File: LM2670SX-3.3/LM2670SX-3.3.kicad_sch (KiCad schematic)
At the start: 2 parts, among them IC1 LM2670SX-3.3_NOPB, J1 Conn_01x03

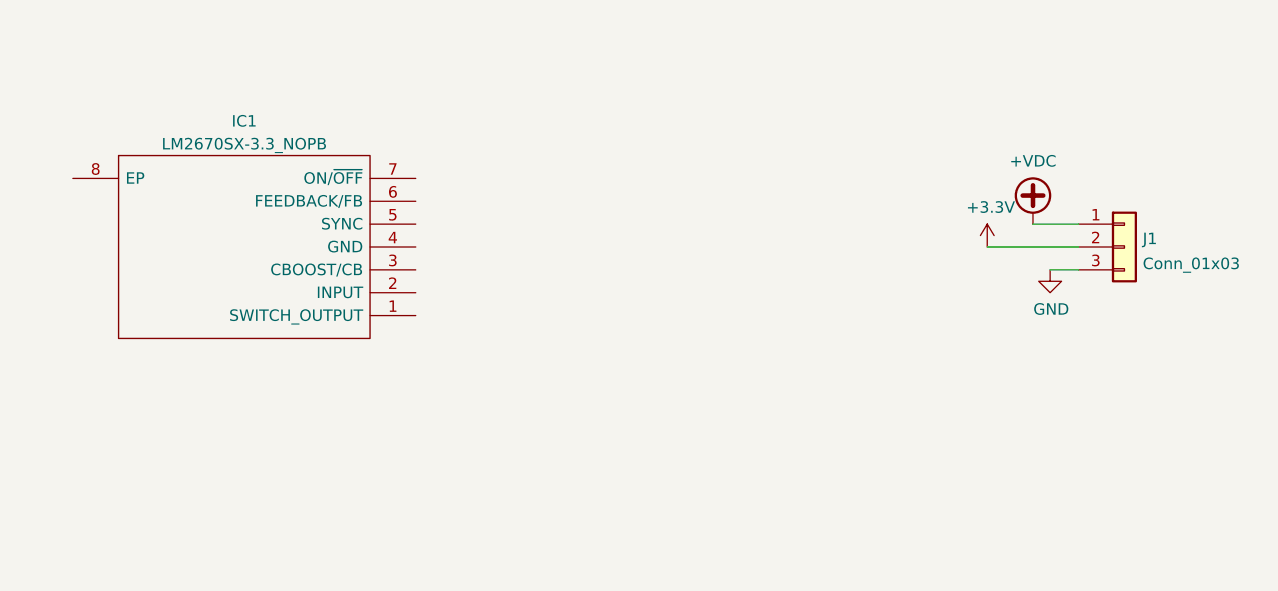
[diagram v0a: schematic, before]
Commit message: finished and drc'ed
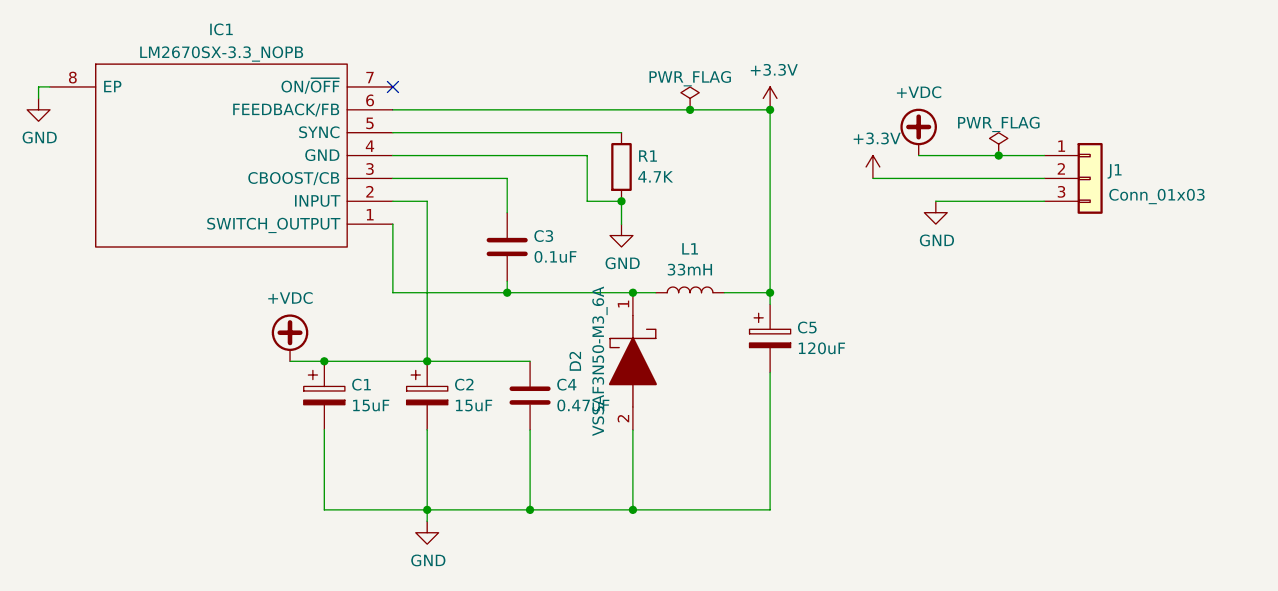
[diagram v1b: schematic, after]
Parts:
- added C1, C2: 15uF, Capacitor_THT:CP_Radial_D5.0mm_P2.50mm, symbol Device:CP
- added C3: 0.1uF, Capacitor_SMD:C_0603_1608Metric_Pad1.08x0.95mm_HandSolder, symbol Device:C
- added C4: 0.47uF, Capacitor_SMD:C_0603_1608Metric_Pad1.08x0.95mm_HandSolder, symbol Device:C
- added C5: 120uF, Capacitor_THT:CP_Radial_D8.0mm_P5.00mm, symbol Device:CP
- added D2: VSSAF3N50-M3_6A, SODFL5226X100N, symbol SamacSys_Parts:VSSAF3N50-M3_6A
- added L1: 33mH, Inductor_THT:L_Axial_L9.5mm_D4.0mm_P15.24mm_Horizontal_Fastron_SMCC, symbol Device:L
- added R1: 4.7K, Resistor_SMD:R_0612_1632Metric_Pad1.18x3.40mm_HandSolder, symbol Device:R
- IC1: footprint LM2670SX33NOPB -> SamacSys_Parts:LM2670SX33NOPB
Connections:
- net +3V3: now also IC1.6 (FEEDBACK/FB), C5.1, L1.2
- net +VDC: now also IC1.2 (INPUT), C1.1, C2.1, C4.1
- net GND: now also IC1.4 (GND), IC1.8 (EP), C1.2, C2.2, C4.2, C5.2, D2.2, R1.2
- net at IC1.1 (SWITCH_OUTPUT): now also C3.2, D2.1, L1.1
- net at IC1.3 (CBOOST/CB): now also C3.1
- net at IC1.5 (SYNC): now also R1.1
- no-connect marks 0 -> 1
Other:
- moved on the sheet: IC1, J1
